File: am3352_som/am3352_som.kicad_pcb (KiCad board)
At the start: 2 copper layers, 2 parts, among them IC1 RTL8211E-VB-CG, J1 SODIMM-204

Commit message: adjust
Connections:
- net GPMC_CSn0 renamed LCD_AC_BIAS_EN
- J1 pad 102: MII1_TXD0 -> MII1_RX_ER
- J1 pad 108: MII1_RX_ER -> MII1_CRS
- J1 pad 127: EXTINTn -> I2C0_SDA
- J1 pad 129: I2C0_SDA -> EXTINTn
- J1 pad 96: MII1_CRS -> MII1_TXD0

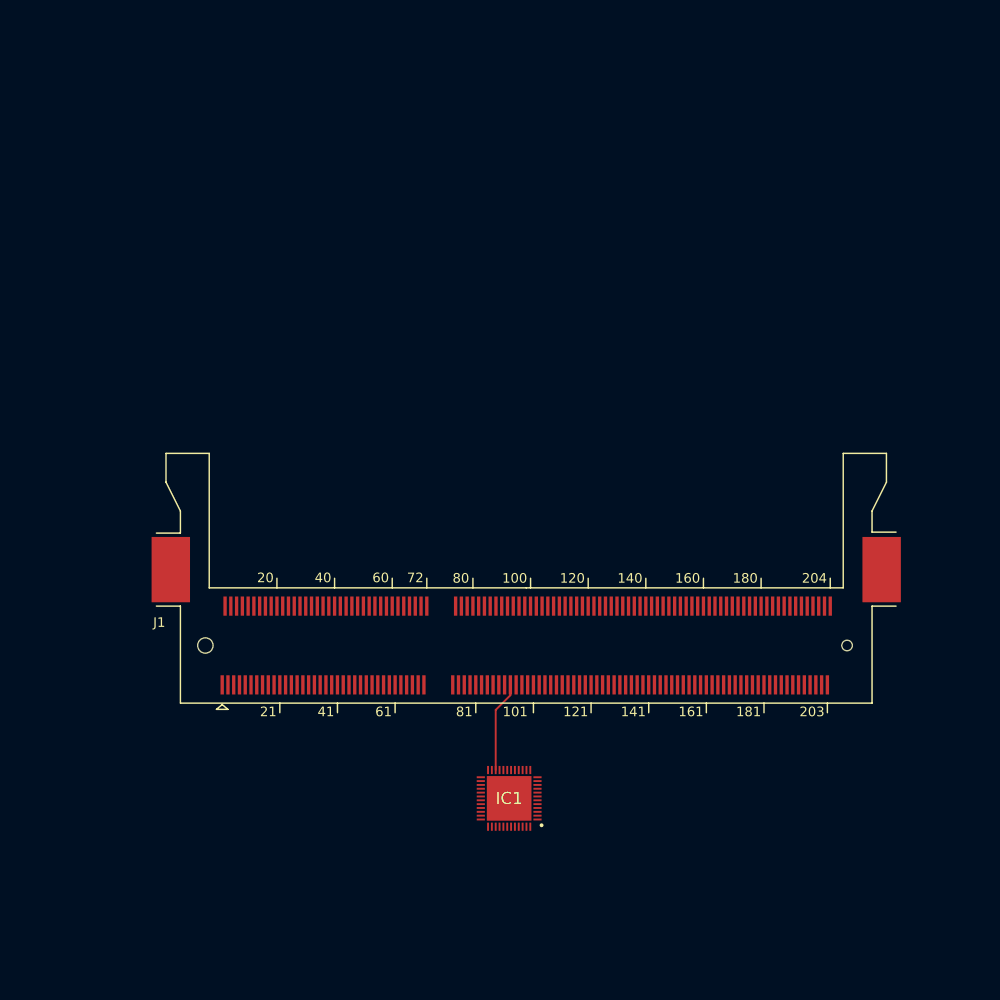
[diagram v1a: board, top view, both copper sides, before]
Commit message: pre
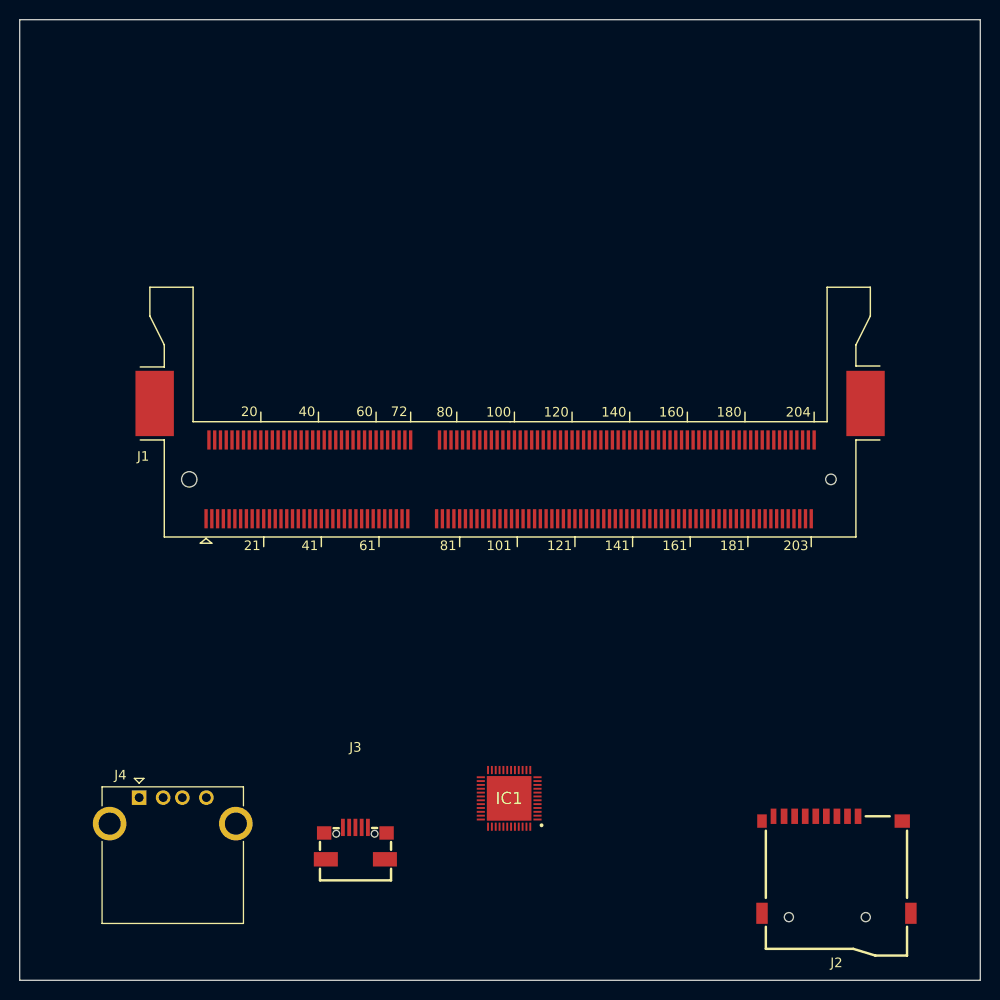
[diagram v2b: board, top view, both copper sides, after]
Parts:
- added J2: Micro_SD_Card, mybays_connector:TFCARD, F.Cu at (185.0, 138.2)
- added J3: microusb, mybays_connector:MICRO-USB_MICRO-USB-17, F.Cu at (134.9, 135.7)
- added J4: USB_A, Connector_USB:USB_A_CONNFLY_DS1095-WNR0, F.Cu at (112.4, 131.0)
- moved J1 17.4 mm to (151.1, 97.9)
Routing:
- net MII1_TX_CLK: track 9.50 -> 0.00 mm
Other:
- board outline added: 100 x 100 mm
